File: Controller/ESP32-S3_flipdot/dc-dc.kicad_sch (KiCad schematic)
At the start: 31 parts, among them J3 BackLight, J5 BL_CMD, J6 BL_PWR, J7 COIL_PWR, Q3 2N3904, Q4 2N3904, Q5 ZXMP4A16G, Q6 ZXMP4A16G, U7 MT3608, U8 MT3608

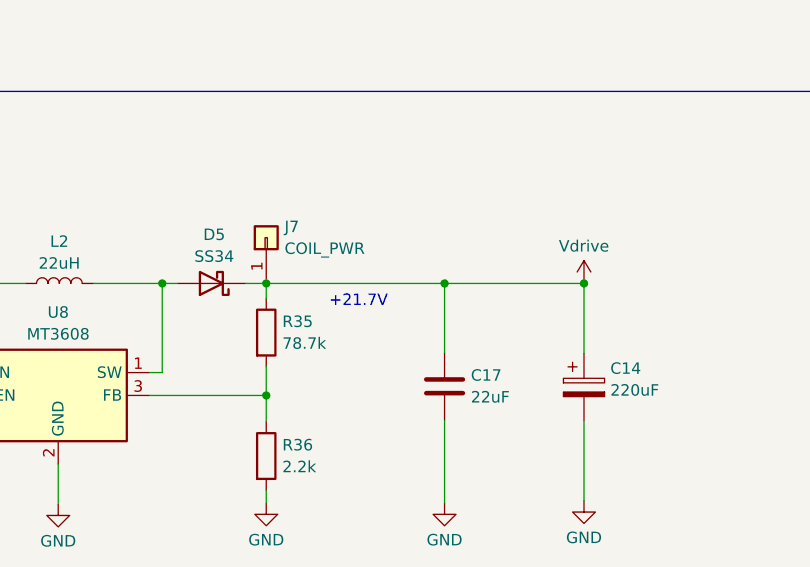
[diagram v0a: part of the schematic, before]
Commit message: Before new dc-dc
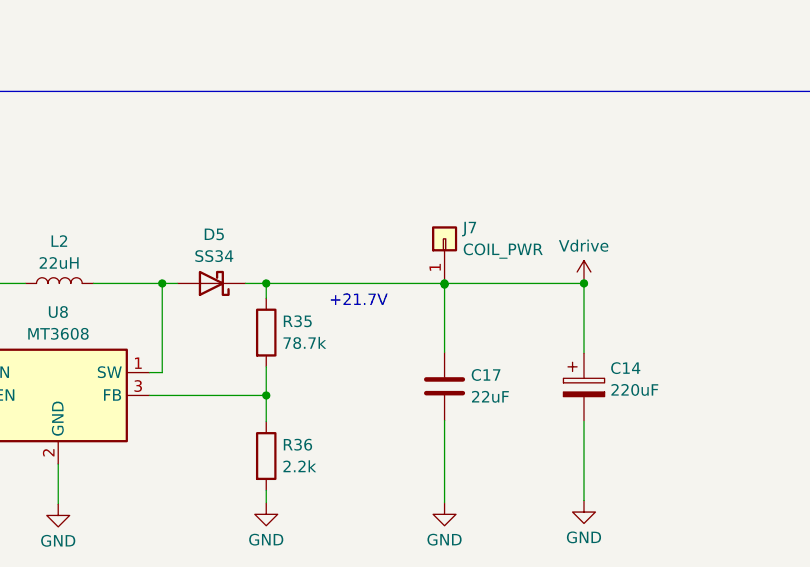
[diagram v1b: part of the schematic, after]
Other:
- moved on the sheet: J7
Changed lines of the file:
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@@
   (junction (at 98.679 144.018) (diameter 0) (color 0 0 0 0)
   )
+  (junction (at 204.343 121.158) (diameter 0) (color 0 0 0 0)
+  )
   (junction (at 217.678 43.815) (diameter 0) (color 0 0 0 0)
   )
@@
     (stroke (width 0) (type default))
   )
-  (wire (pts (xy 204.343 121.031) (xy 204.343 128.651))
-    (stroke (width 0) (type default))
-  )
   (wire (pts (xy 118.999 109.347) (xy 103.759 109.347))
     (stroke (width 0) (type default))
@@
     (stroke (width 0) (type default))
   )
+  (wire (pts (xy 204.343 121.158) (xy 204.343 128.651))
+    (stroke (width 0) (type default))
+  )
   (wire (pts (xy 228.473 54.483) (xy 227.838 54.483))
     (stroke (width 0) (type default))
@@
   )
   (wire (pts (xy 81.915 128.778) (xy 85.217 128.778))
+    (stroke (width 0) (type default))
+  )
+  (wire (pts (xy 204.343 121.158) (xy 204.343 121.031))
     (stroke (width 0) (type default))
   )
@@
     )
   )
-  (symbol (lib_id "Connector_Generic:Conn_01x01") (at 184.531 115.951 90) (unit 1)
-    (in_bom yes) (on_board yes) (dnp no) (fields_autoplaced)
-    (property "Reference" "J7" (at 186.563 114.7389 90)
+  (symbol (lib_id "Connector_Generic:Conn_01x01") (at 204.343 116.078 90) (unit 1)
+    (in_bom yes) (on_board yes) (dnp no) (fields_autoplaced)
+    (property "Reference" "J7" (at 206.375 114.8659 90)
       (effects (font (size 1.27 1.27)) (justify right))
     )
-    (property "Value" "COIL_PWR" (at 186.563 117.1631 90)
+    (property "Value" "COIL_PWR" (at 206.375 117.2901 90)
       (effects (font (size 1.27 1.27)) (justify right))
     )
-    (property "Footprint" "TestPoint:TestPoint_THTPad_2.0x2.0mm_Drill1.0mm" (at 184.531 115.951 0)
-      (effects (font (size 1.27 1.27)) hide)
-    )
-    (property "Datasheet" "~" (at 184.531 115.951 0)
-      (effects (font (size 1.27 1.27)) hide)
-    )
+    (property "Footprint" "TestPoint:TestPoint_THTPad_2.0x2.0mm_Drill1.0mm" (at 204.343 116.078 0)
+      (effects (font (size 1.27 1.27)) hide)
+    )
+    (property "Datasheet" "~" (at 204.343 116.078 0)
+      (effects (font (size 1.27 1.27)) hide)
+    )
